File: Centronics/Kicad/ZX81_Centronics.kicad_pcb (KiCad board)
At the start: 2 copper layers, 68.8 x 91.4 mm, 19 parts, among them J1 CENTRONICS, Q1 BC558, SW1 SW_Push, U1 74LS27, U2 74LS32, U3 74LS30, U4 8255

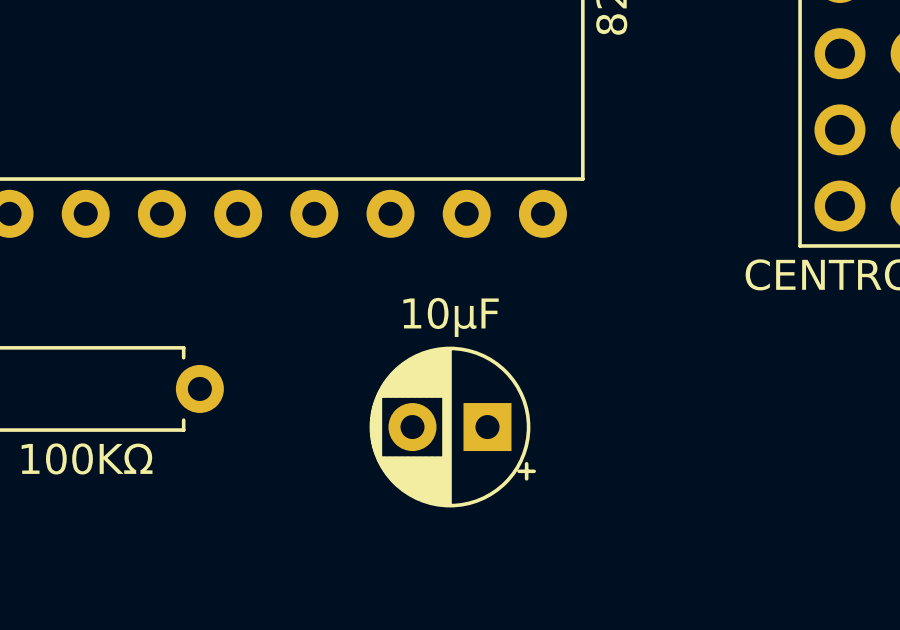
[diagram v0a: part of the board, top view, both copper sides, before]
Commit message: Updated schematic plot
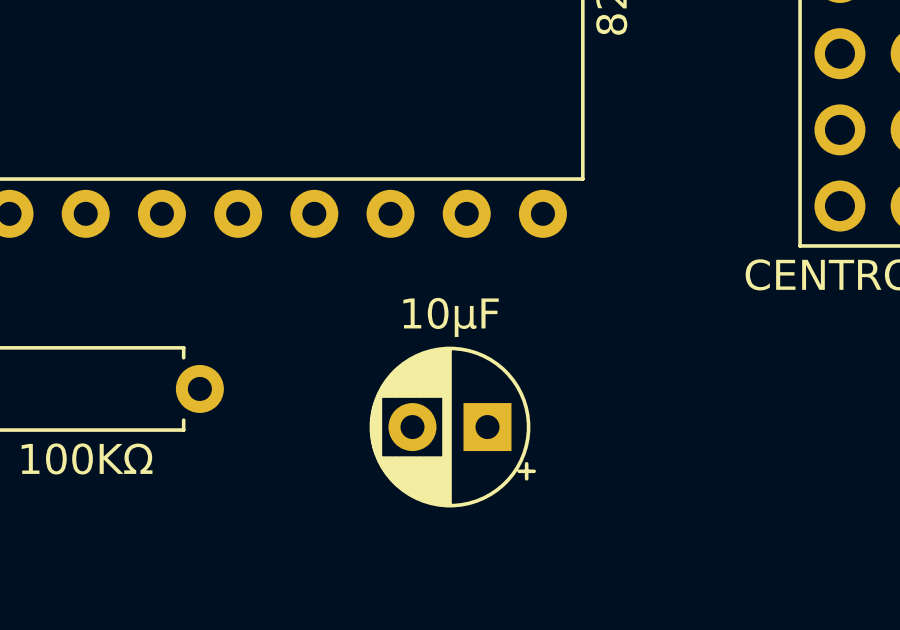
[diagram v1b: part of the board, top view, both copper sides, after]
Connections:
- BUS1 pad GND: (no net) -> GND
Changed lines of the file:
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@@
   )
   (footprint "Capacitor_THT:CP_Radial_D5.0mm_P2.50mm" (layer "F.Cu")
-    (at 145.477113 99.314 180)
+    (at 145.4771 99.314 180)
     (descr "CP, Radial series, Radial, pin pitch=2.50mm, , diameter=5mm, Electrolytic Capacitor")
     (tags "CP Radial series Radial pin pitch 2.50mm  diameter 5mm Electrolytic Capacitor")
@@
     (pad "23B" connect rect (at 20.955 -7.747) (size 1.778 7.62) (layers "B.Cu" "B.Mask")
       (net 31 "/~{ROMCS}") (pinfunction "~{ROM_CS}") (pintype "output"))
-    (pad "GND" connect rect (at -25.9715 -5.9055) (size 2.99974 4.0005) (layers "B.Cu" "B.Mask"))
+    (pad "GND" connect rect (at -25.9715 -5.9055) (size 2.99974 4.0005) (layers "B.Cu" "B.Mask")
+      (net 14 "GND"))
   )
   (gr_line (start 163.83 121.158) (end 152.908 121.158)
